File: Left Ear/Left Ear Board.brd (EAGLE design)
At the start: 33 x 32.4 mm, 23 parts

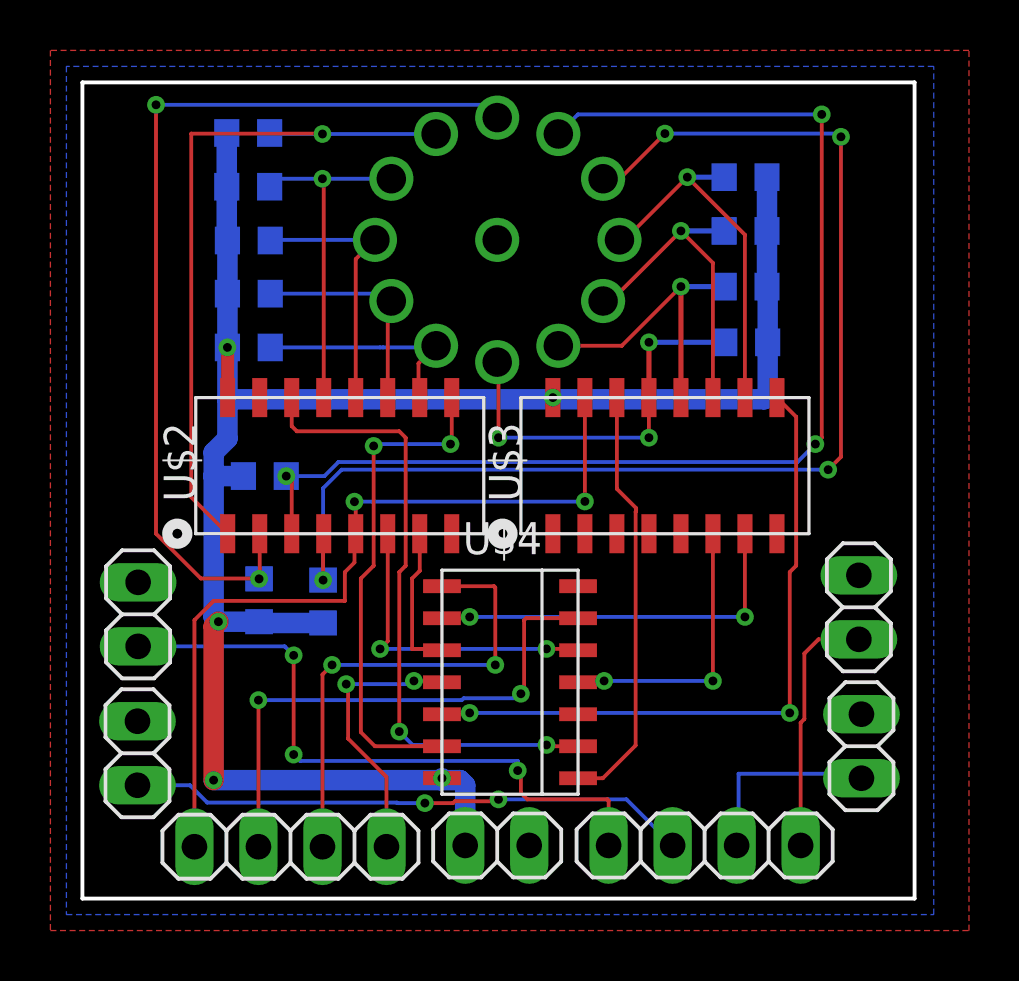
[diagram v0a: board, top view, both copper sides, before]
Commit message: Worked on code
Updated board layouts since shit changed
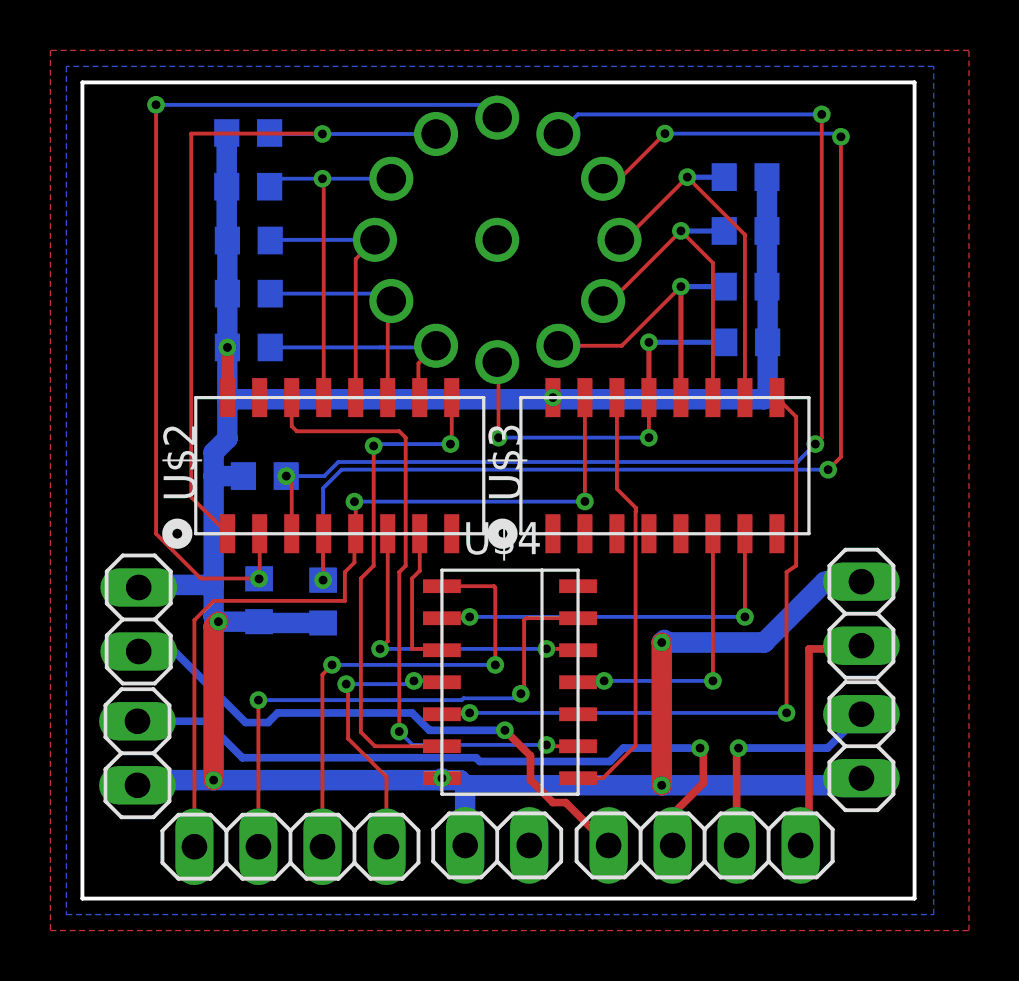
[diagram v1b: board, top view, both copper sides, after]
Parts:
- moved JP6 0.27 mm to (30.9, 11.3), turned to 270 degrees
- moved JP3 0.20 mm to (2.24, 11.1), turned to 270 degrees
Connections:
- net GND: no longer JP3.2, JP4.2, JP5.2, JP6.2
- net N$21: now also JP3.2; no longer JP3.1
- net N$22: now also JP4.2; no longer JP4.1
- net N$23: now also JP5.2; no longer JP5.1
- net N$24: now also JP6.2; no longer JP6.1
- net VCC: now also JP3.1, JP4.1, JP5.1, JP6.1
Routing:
- net VCC: track 76.2 -> 112.9 mm, vias 5 -> 7
- net N$22: track 22.3 -> 27.6 mm, vias 2 -> 1
- net N$21: track 26.0 -> 22.7 mm, vias 3 -> 1
- net N$23: track 7.83 -> 9.33 mm, vias 0 -> 1
- net N$24: track 10.1 -> 10.7 mm

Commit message: Fix
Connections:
- net GND: now also U$3.5
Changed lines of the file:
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@@
 <?xml version="1.0" encoding="utf-8"?>
 <!DOCTYPE eagle SYSTEM "eagle.dtd">
-<eagle version="8.6.1">
+<eagle version="8.6.3">
 <drawing>
 <settings>
@@
 <vertex x="33.782" y="33.02"/>
 </polygon>
+<contactref element="U$3" pad="5"/>
 </signal>
 <signal name="N$1">
